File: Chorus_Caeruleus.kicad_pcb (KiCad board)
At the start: 2 copper layers, 55 x 80 mm, 125 parts, among them Q1 2N5088, Q10 J201, Q11 J201, Q2 2N5088, Q3 2N5088, Q4 2N5088, Q5 2N5088, Q7 2SC1815, Q8 2SC1815, Q9 2SC1815, SW1 SW_Push, SW2 SW_SPST, U1 RC4558, U2 MN3207, U3 MN3102, U4 TL022

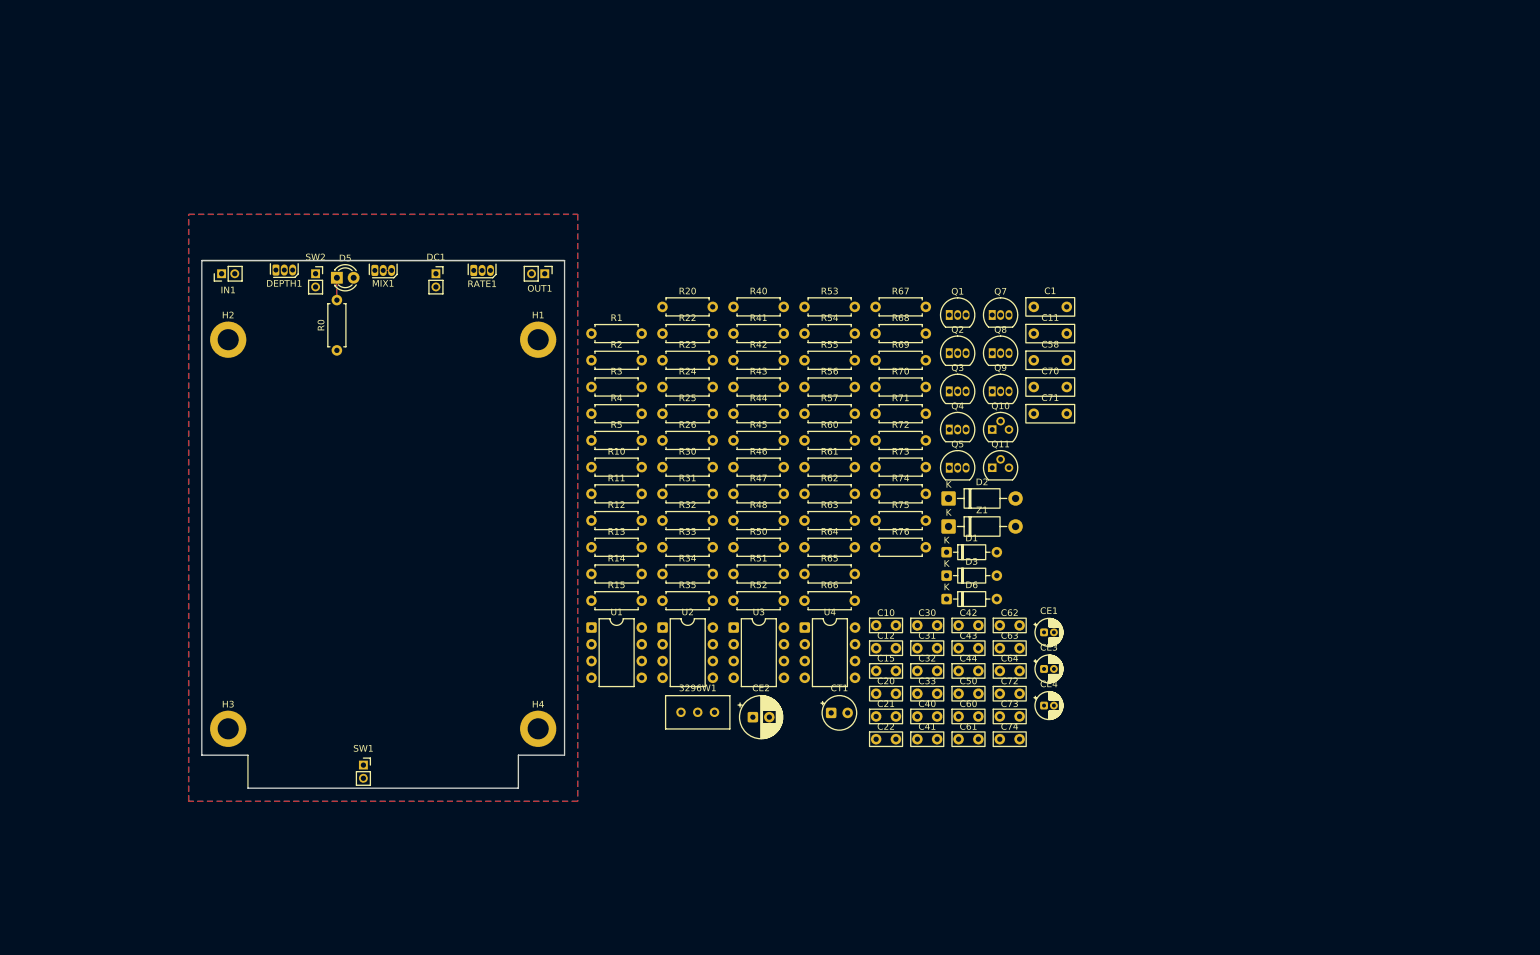
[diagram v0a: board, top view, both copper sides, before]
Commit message: Proj renamed, PCB upd
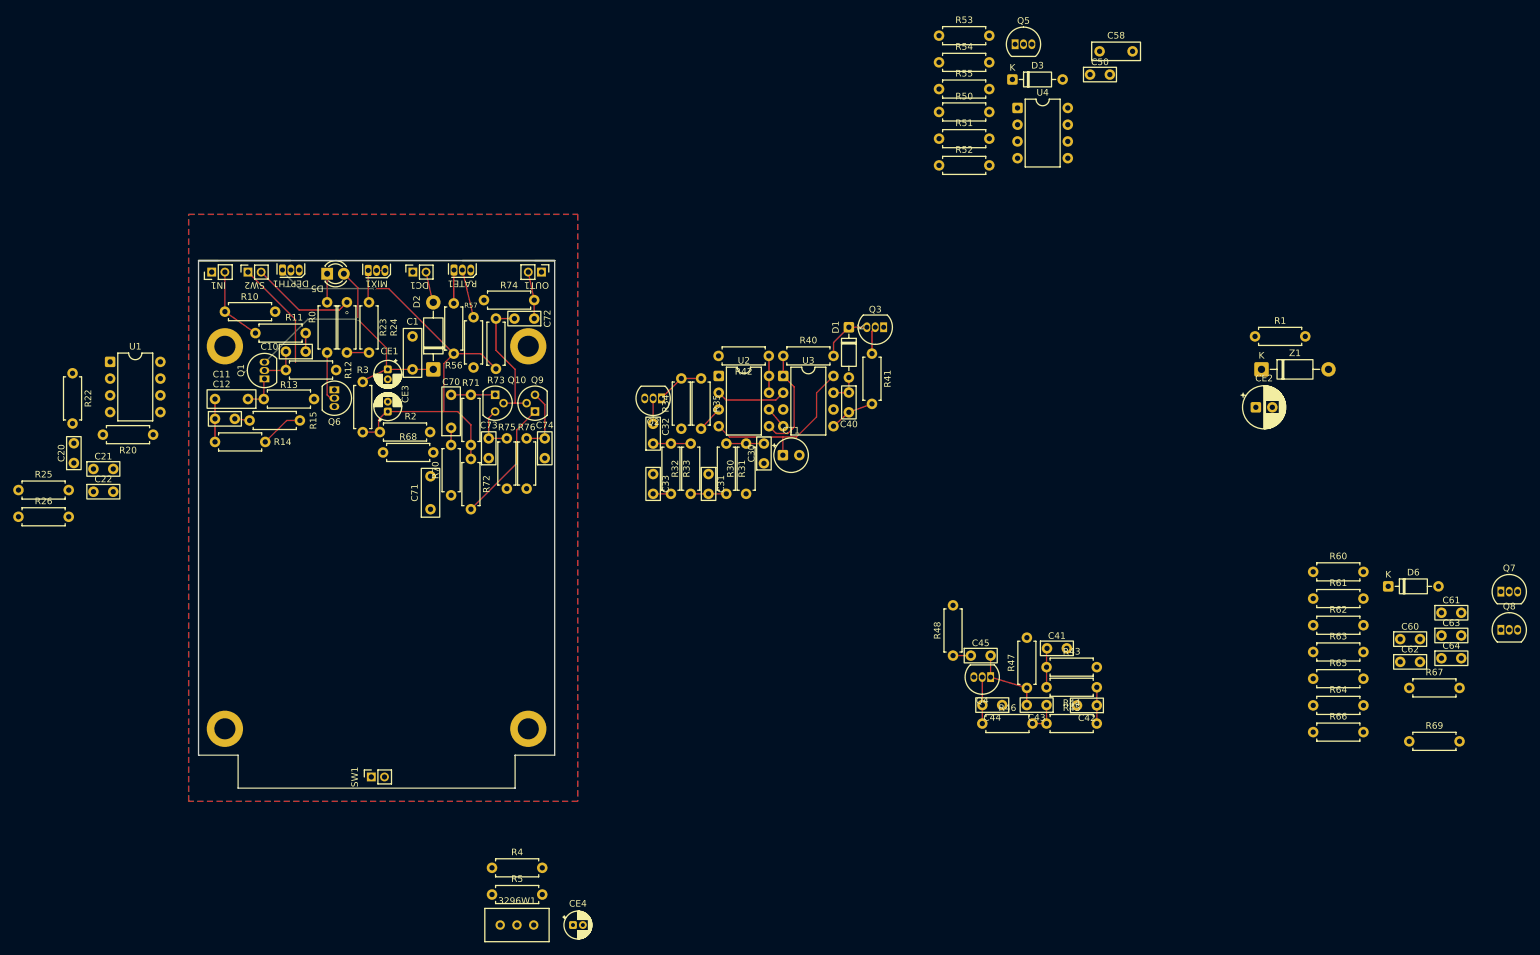
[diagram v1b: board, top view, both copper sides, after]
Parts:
- moved C20 126.6 mm to (60.6, 90.7), turned to 90 degrees
- moved C21 124.5 mm to (63.6, 91.6)
- moved C22 124.5 mm to (63.6, 95.0)
- moved C11 119.6 mm to (87.0, 81.0), turned to 180 degrees
- moved CE1 107.2 mm to (108.2, 76.5), turned to -90 degrees
- moved CE3 106.9 mm to (108.2, 82.9), turned to 90 degrees
- moved C12 106.1 mm to (82.0, 84.0)
- moved Q1 104.3 mm to (89.5, 77.9), turned to 90 degrees
- moved R1 100.6 mm to (239.7, 71.5)
- moved Q6 99.7 mm to (100.1, 79.6), turned to -90 degrees
- moved R69 99.4 mm to (263.1, 132.9)
- moved R67 99.4 mm to (263.1, 124.8)
- moved R25 98.3 mm to (52.2, 94.8)
- moved R26 98.3 mm to (52.2, 98.8)
- moved C50 96.0 mm to (214.7, 31.8)
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- renumbered C15 to C44, C44 to C45, C62 to C61, C61 to C62, Q5 to Q2, Q2 to Q5, Q9 to Q6, Q11 to Q9, R65 to R64, R64 to R65
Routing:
- net /VC: track 0.00 -> 73.9 mm, vias 0 -> 1
- net /VA: track 0.00 -> 45.5 mm, vias 0 -> 1
- net Net-(U2-VGG): track 0.00 -> 26.8 mm
- net Net-(Q10-S): track 0.00 -> 20.3 mm
- net Net-(Q10-D): track 0.00 -> 18.8 mm
- net /RC_OUT: track 0.00 -> 16.7 mm
- net /VD: track 0.00 -> 16.2 mm
- net Net-(SW2-B): track 0.00 -> 15.9 mm
- net /IN: track 0.00 -> 11.7 mm
- net /Q4_1: track 0.00 -> 11.6 mm
- net Net-(U2-CP1): track 0.00 -> 10.7 mm
- net Net-(Q10-G): track 0.00 -> 9.97 mm
- net Net-(D1-K): track 0.00 -> 8.05 mm
- net Net-(Q6-C): track 0.00 -> 7.73 mm
- net Net-(R57-Pad1): track 0.00 -> 7.36 mm
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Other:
- board size 55 x 80 mm -> 54 x 80 mm
- board text added: "DC1"
- board text added: "DEPTH1"
- board text added: "IN1"
- board text added: "MIX1"
- board text added: "OUT1"
- board text added: "RATE1"
- board text added: "SW2"

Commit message: PCB upd
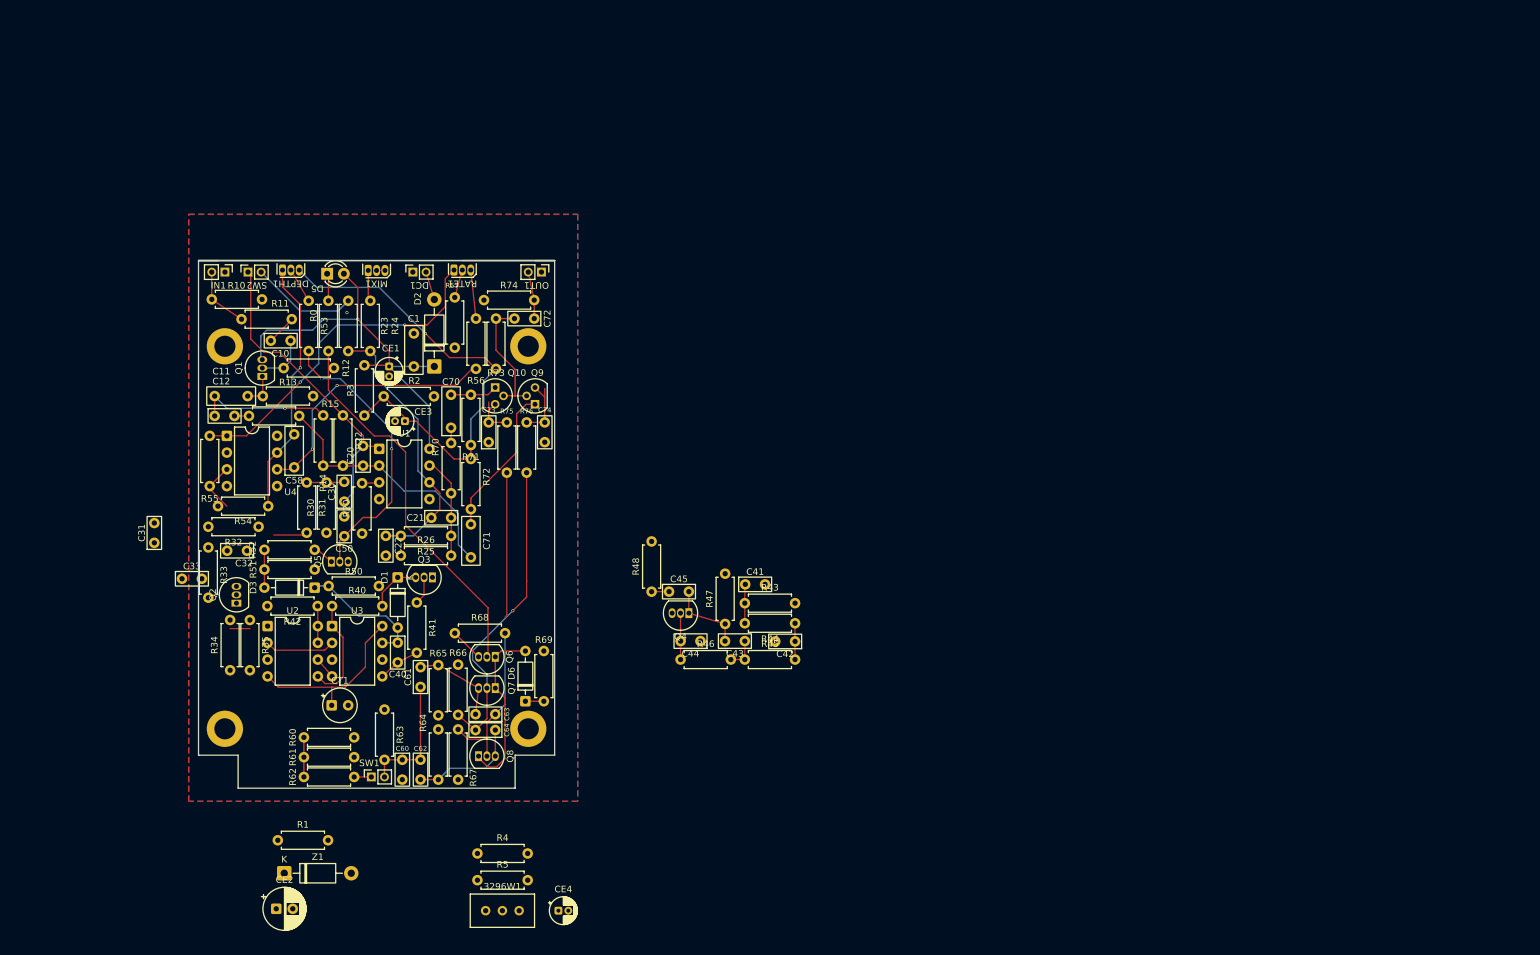
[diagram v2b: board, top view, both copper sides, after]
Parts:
- moved CE2 166.9 mm to (91.3, 158.3)
- moved R1 166.7 mm to (91.5, 147.9)
- moved Z1 166.7 mm to (92.5, 152.9)
- moved Q8 156.2 mm to (122.0, 135.2)
- moved C61 155.2 mm to (113.2, 124.7), turned to 90 degrees
- moved Q7 153.2 mm to (124.5, 124.8), turned to 180 degrees
- moved C60 152.4 mm to (110.4, 135.7), turned to -90 degrees
- moved C62 149.3 mm to (113.2, 135.7), turned to -90 degrees
- moved R60 147.6 mm to (103.1, 132.3), turned to 180 degrees
- moved R61 147.4 mm to (103.1, 135.3), turned to 180 degrees
- moved R62 147.2 mm to (103.1, 138.3), turned to 180 degrees
- moved R67 144.9 mm to (118.9, 138.7), turned to 90 degrees
- moved C63 144.0 mm to (124.5, 128.8), turned to 180 degrees
- moved C64 143.9 mm to (124.5, 131.2), turned to 180 degrees
- moved R63 141.1 mm to (107.7, 128.1), turned to -90 degrees
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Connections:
- DEPTH1 pad 1: /VC -> Net-(C58-Pad2)
- DEPTH1 pad 3: Net-(C58-Pad2) -> /VC
- R71 pad 1: /VC -> Net-(Q9-D)
- R71 pad 2: Net-(Q9-D) -> /VC
- RATE1 pad 1: Net-(R56-Pad1) -> Net-(R55-Pad2)
- RATE1 pad 3: Net-(R55-Pad2) -> Net-(R56-Pad1)
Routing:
- net Net-(R55-Pad2): track 0.00 -> 52.0 mm, vias 0 -> 2
- net Net-(Q6-C): track 7.73 -> 57.8 mm
- net /OFF: track 0.00 -> 47.5 mm, vias 0 -> 1
- net /ON: track 0.00 -> 46.8 mm
- net Net-(Q5-B): track 0.00 -> 43.2 mm, vias 0 -> 2
- net Net-(U4B--): track 0.00 -> 39.6 mm, vias 0 -> 2
- net Net-(C58-Pad2): track 0.00 -> 39.4 mm, vias 0 -> 1
- net /U1_6: track 3.35 -> 41.5 mm
- net /PR_IN: track 6.60 -> 40.4 mm
- net /RC_OUT: track 16.7 -> 47.5 mm
- net Net-(D6-A): track 0.00 -> 26.3 mm
- net Net-(C60-Pad1): track 0.00 -> 18.7 mm
- net Net-(Q8-B): track 0.00 -> 17.0 mm
- net /VA: track 45.5 -> 62.3 mm
- net /LFO: track 4.63 -> 19.8 mm
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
